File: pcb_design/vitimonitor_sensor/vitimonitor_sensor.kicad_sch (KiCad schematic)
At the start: 26 parts, among them J1 USB_C_Receptacle_USB2.0_14P, SW1 BOOT, SW2 RESETN, U1 ESP32-C3-WROOM-02U, U2 USBLC6-2SC6, U3 LM1117DT-3.3

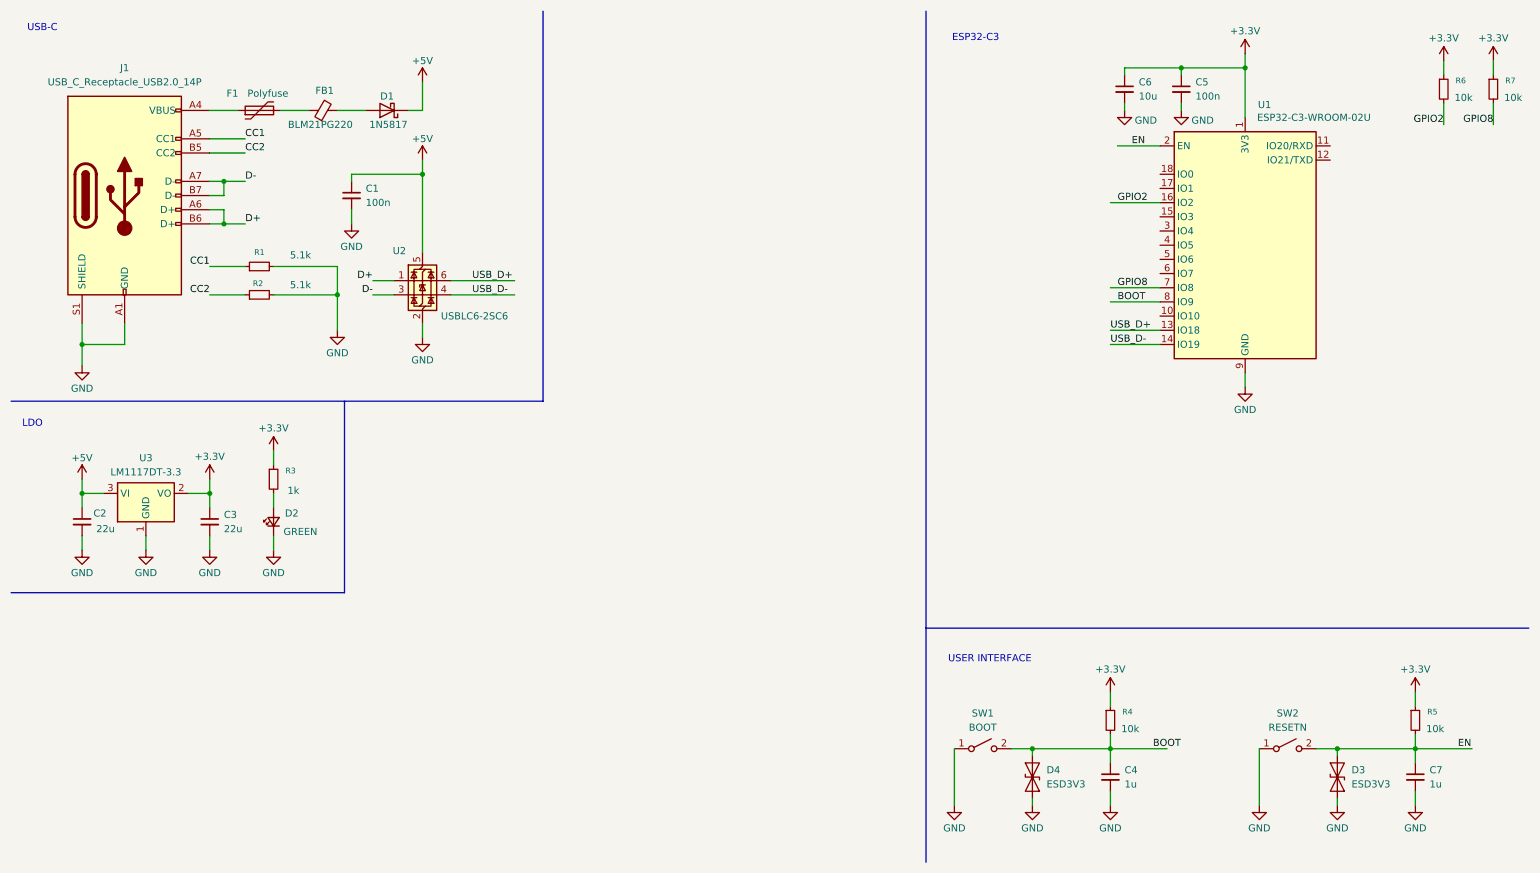
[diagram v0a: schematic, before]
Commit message: Kicad Schematic Update
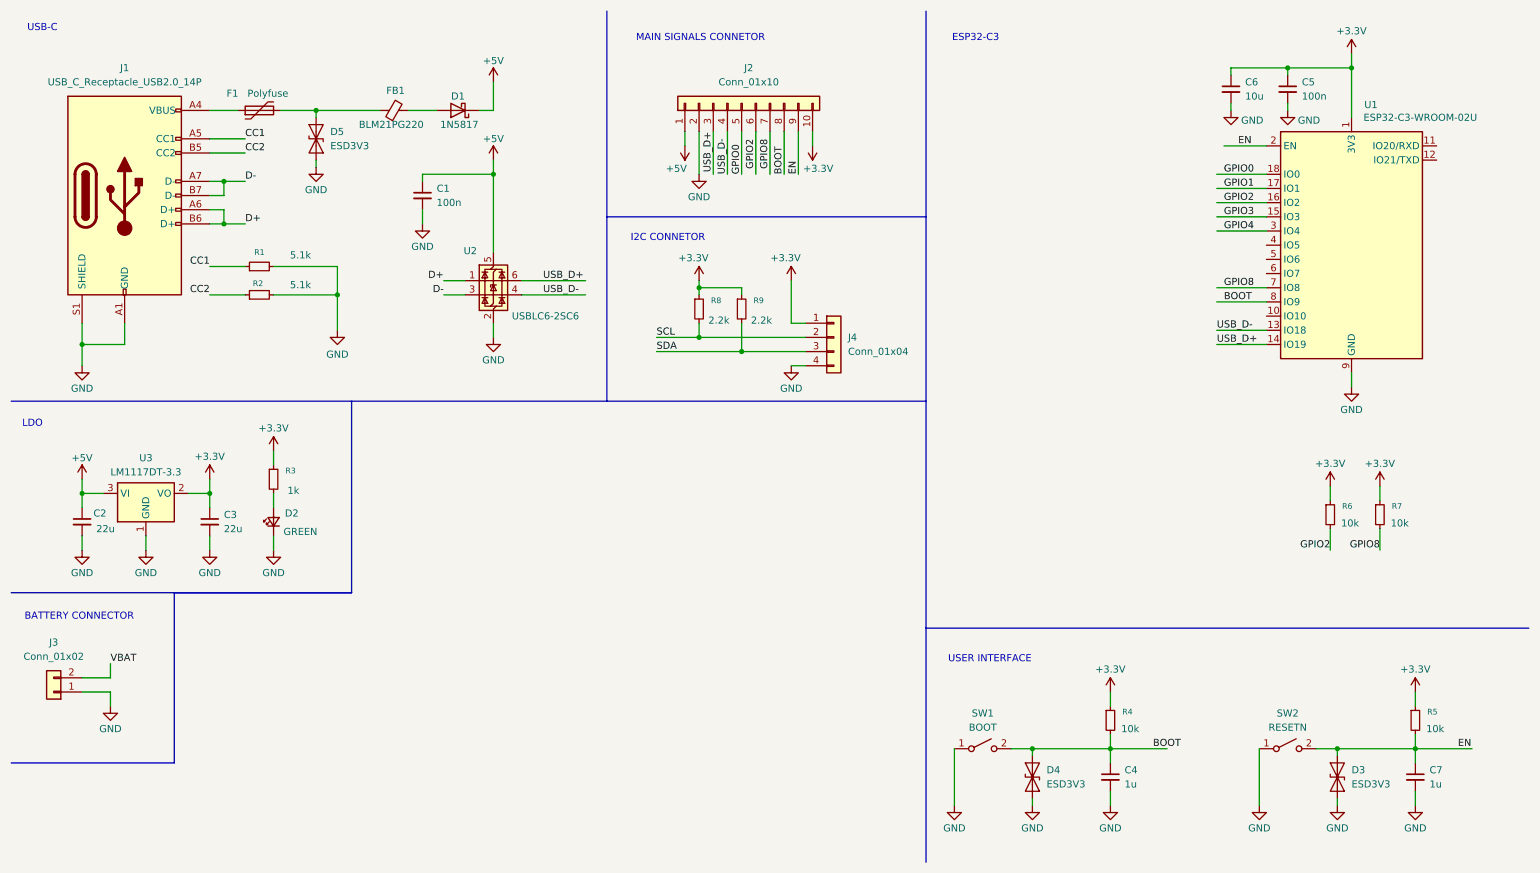
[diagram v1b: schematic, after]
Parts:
- added D5: ESD3V3, Diode_SMD:D_SOD-923, symbol Diode:ESD9B3.3ST5G
- added J2: Conn_01x10, symbol Connector_Generic:Conn_01x10
- added J3: Conn_01x02, symbol Connector_Generic:Conn_01x02
- added J4: Conn_01x04, symbol Connector_Generic:Conn_01x04
- added R8, R9: 2.2k, symbol Device:R_Small
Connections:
- net +3.3V: now also J2.10 (Pin_10), J4.1 (Pin_1), R8.1, R9.1
- net +5V: now also J2.1 (Pin_1)
- net BOOT: now also J2.8 (Pin_8)
- net EN: now also J2.9 (Pin_9)
- net GND: now also D5.1 (A1), J2.2 (Pin_2), J3.1 (Pin_1), J4.4 (Pin_4)
- net GPIO2: now also J2.6 (Pin_6)
- net GPIO8: now also J2.7 (Pin_7)
- net USB_D+: now also U1.14 (IO19), J2.3 (Pin_3); no longer U1.13 (IO18)
- net USB_D-: now also U1.13 (IO18), J2.4 (Pin_4); no longer U1.14 (IO19)
- net at F1.2, FB1.1: now also D5.2 (A2)
- net GPIO3: now reaches U1.15 (IO3)
- net GPIO1: now reaches U1.17 (IO1)
- net GPIO0: now reaches U1.18 (IO0)
- net GPIO0: now also J2.5 (Pin_5)
- net GPIO4: now reaches U1.3 (IO4)
- new net SCL: J4.2 (Pin_2), R8.2
- new net SDA: J4.3 (Pin_3), R9.2
- new net VBAT: J3.2 (Pin_2)
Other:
- note added: "BATTERY CONNECTOR"
- note added: "I2C CONNETOR"
- note added: "MAIN SIGNALS CONNETOR"
- moved on the sheet: C1, C5, C6, D1, FB1, R6, R7, U1, U2
